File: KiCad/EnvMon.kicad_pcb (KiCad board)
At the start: 2 copper layers, 44.5 x 37 mm, 14 parts, among them J1 DS18B20, J2 Prog, J3 12V, J4 USB-C, M1 SCD30, M2 OLED1.5-I2C, M3 D24V5F3, SW1 GPIO0, U1 ESP32-WROOM-32

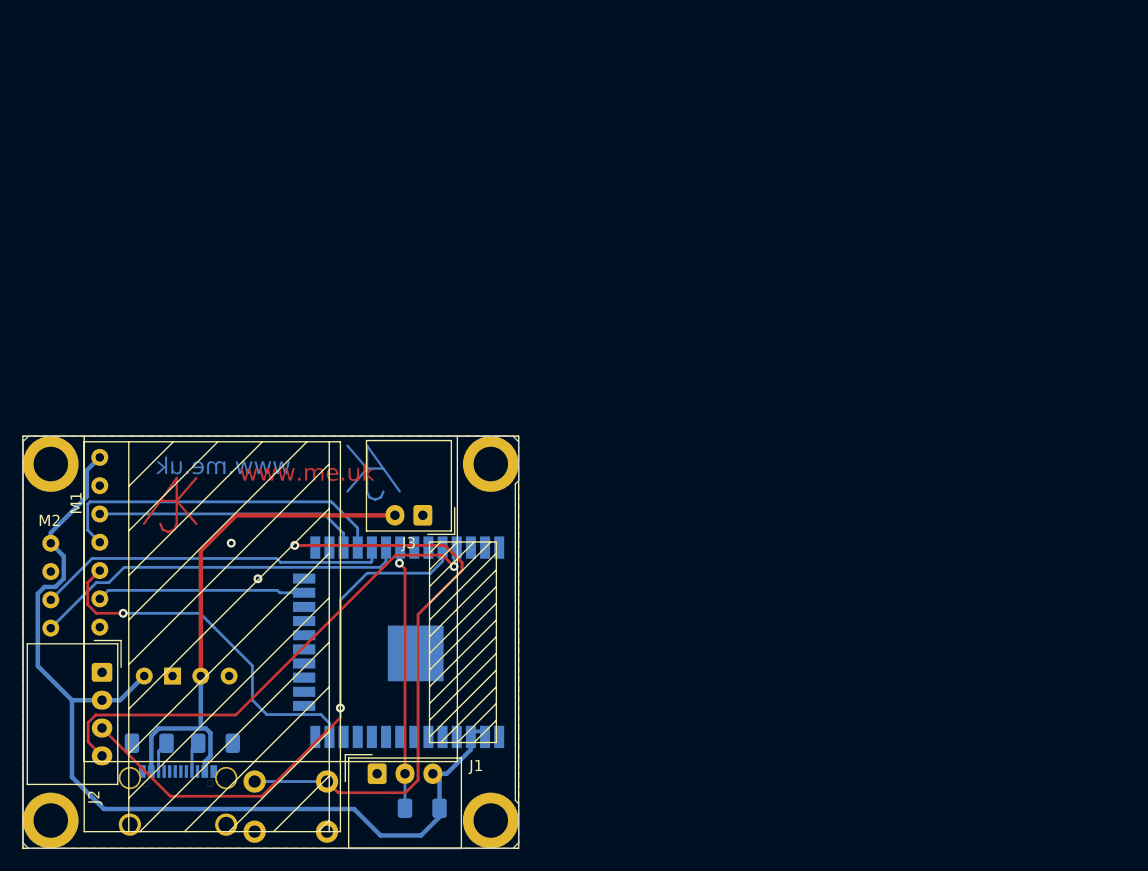
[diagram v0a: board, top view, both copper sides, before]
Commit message: Updated
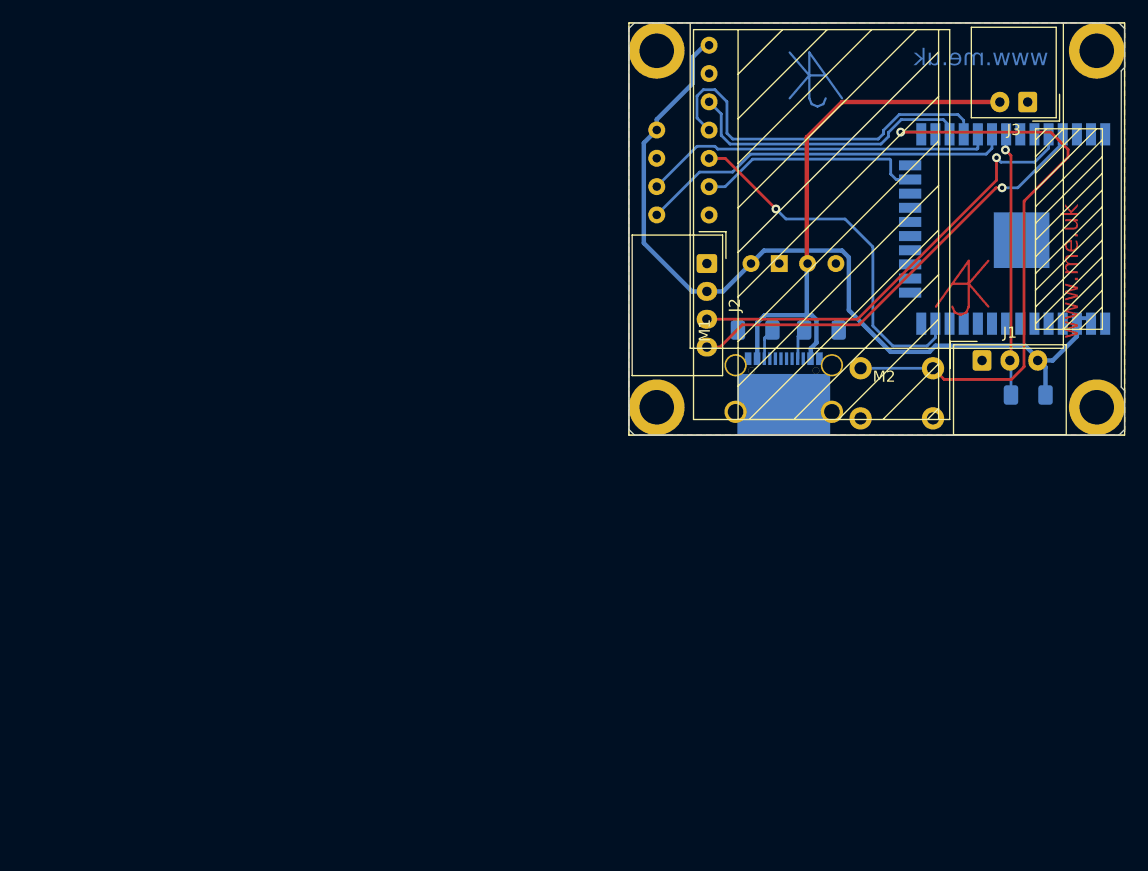
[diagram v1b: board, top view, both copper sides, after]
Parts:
- moved REF** 73.7 mm to (150.9, 106.1)
- moved M1 66.0 mm to (125.7, 114.0)
- moved M3 65.9 mm to (134.7, 101.3)
- moved R1 65.8 mm to (155.8, 111.8)
- moved M2 65.8 mm to (164.4, 78.4)
- moved R2 65.8 mm to (131.2, 106.0)
- moved R3 65.8 mm to (137.2, 106.0)
- moved SW1 65.8 mm to (147.2, 109.4)
- moved U1 65.8 mm to (154.4, 96.9)
- moved J4 65.8 mm to (133.8, 115.4)
- moved J1 65.8 mm to (151.6, 108.7)
- moved J3 65.8 mm to (155.7, 85.5)
- moved J2 65.5 mm to (126.9, 100.0)
- moved REF** 53.1 mm to (135.6, 87.4)
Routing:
- net +3V3: track 89.1 -> 77.6 mm
- net Net-(J2-Pad3): track 49.8 -> 39.8 mm
- net Net-(J2-Pad4): track 45.3 -> 40.7 mm
- net Net-(M1-Pad4): track 30.4 -> 33.7 mm
- net Net-(M1-Pad3): track 23.4 -> 26.4 mm
- net Net-(M1-Pad6): track 18.8 -> 20.6 mm
- net /VBUS: track 48.0 -> 47.4 mm
- net GND: vias 2 -> 0
